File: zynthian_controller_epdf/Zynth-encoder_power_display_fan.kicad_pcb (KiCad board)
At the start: 2 copper layers, 65 x 56 mm, 42 parts, among them J3 40HAT, Q1 DMG2305UX, Q2 DMMT5401, Q3 Q_NMOS_GDS, U2 CAT24C32, U3 MCP23017_SS

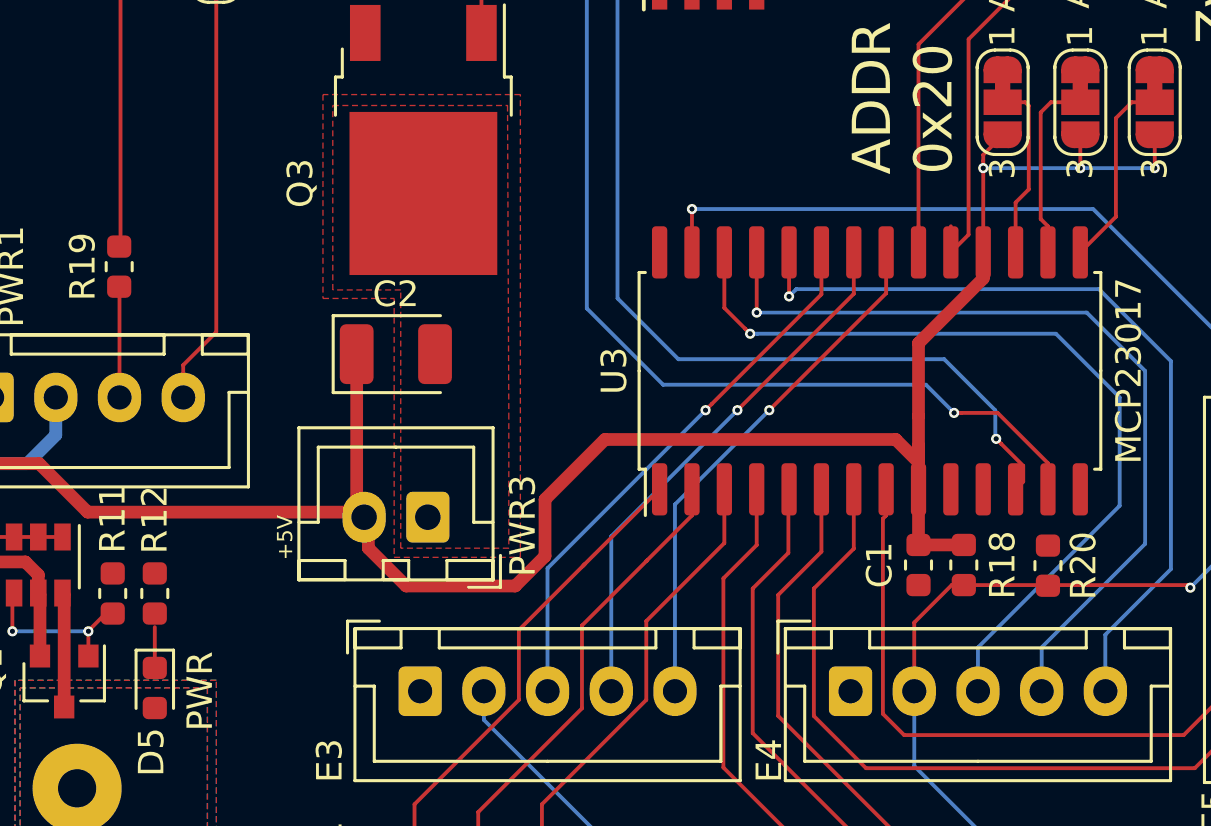
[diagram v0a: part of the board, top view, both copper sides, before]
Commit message: Submit to MFG
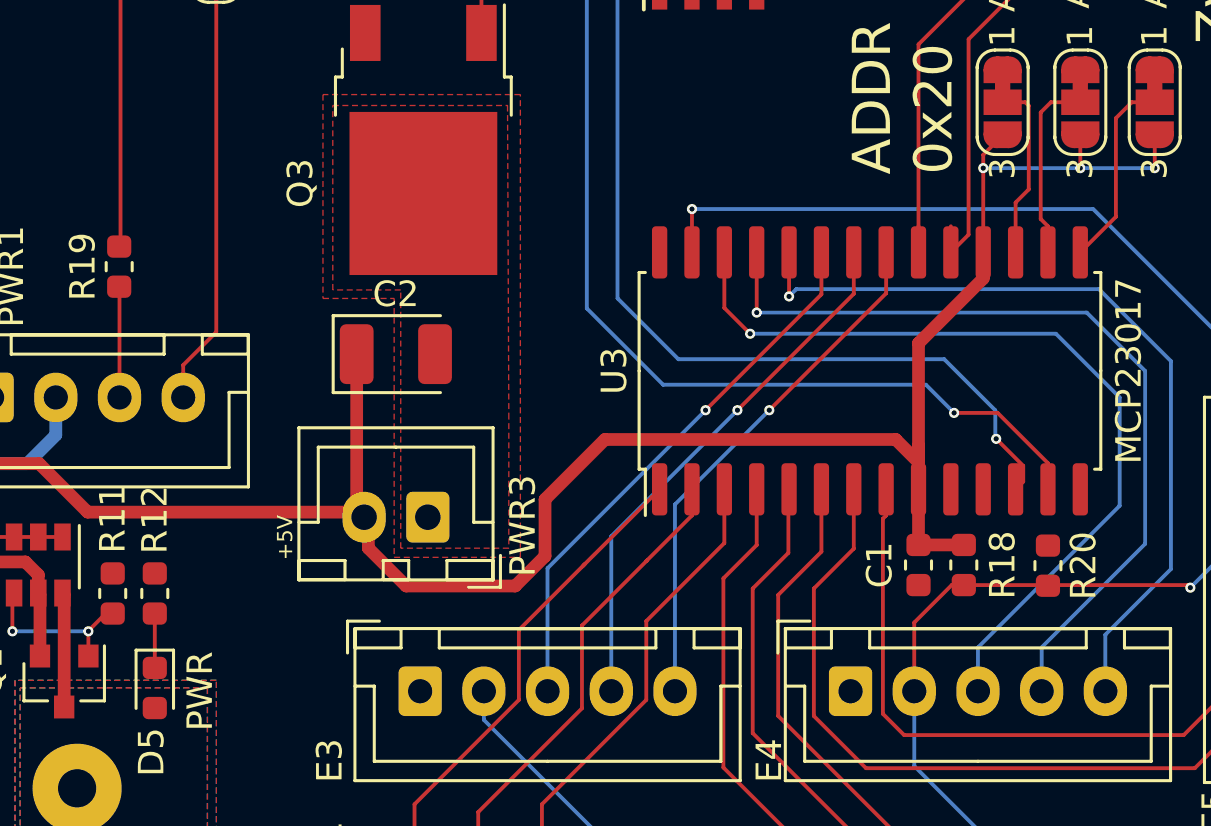
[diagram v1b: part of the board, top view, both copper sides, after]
